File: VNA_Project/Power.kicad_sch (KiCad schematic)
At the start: 33 parts, among them J201 USB_C_Receptacle_USB2.0_16P, J202 Jack-DC, U201 AP7375, U202 USBLC6-2SC6, U203 TLV62569DBV, U204 HT7533-1

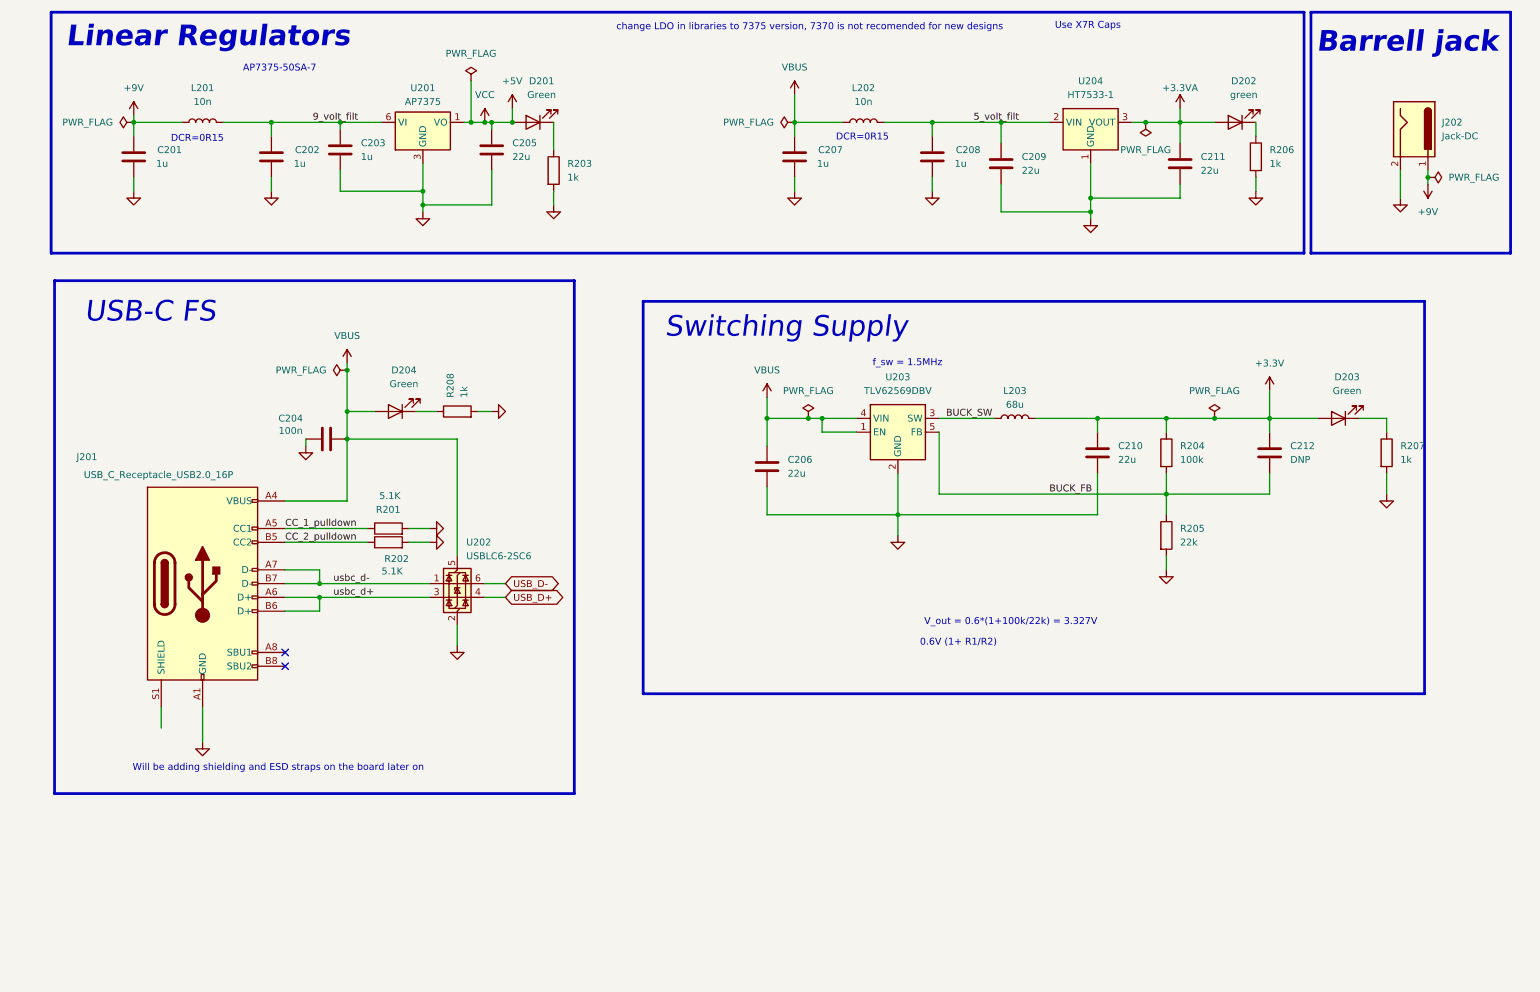
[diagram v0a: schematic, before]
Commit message: adc
adc
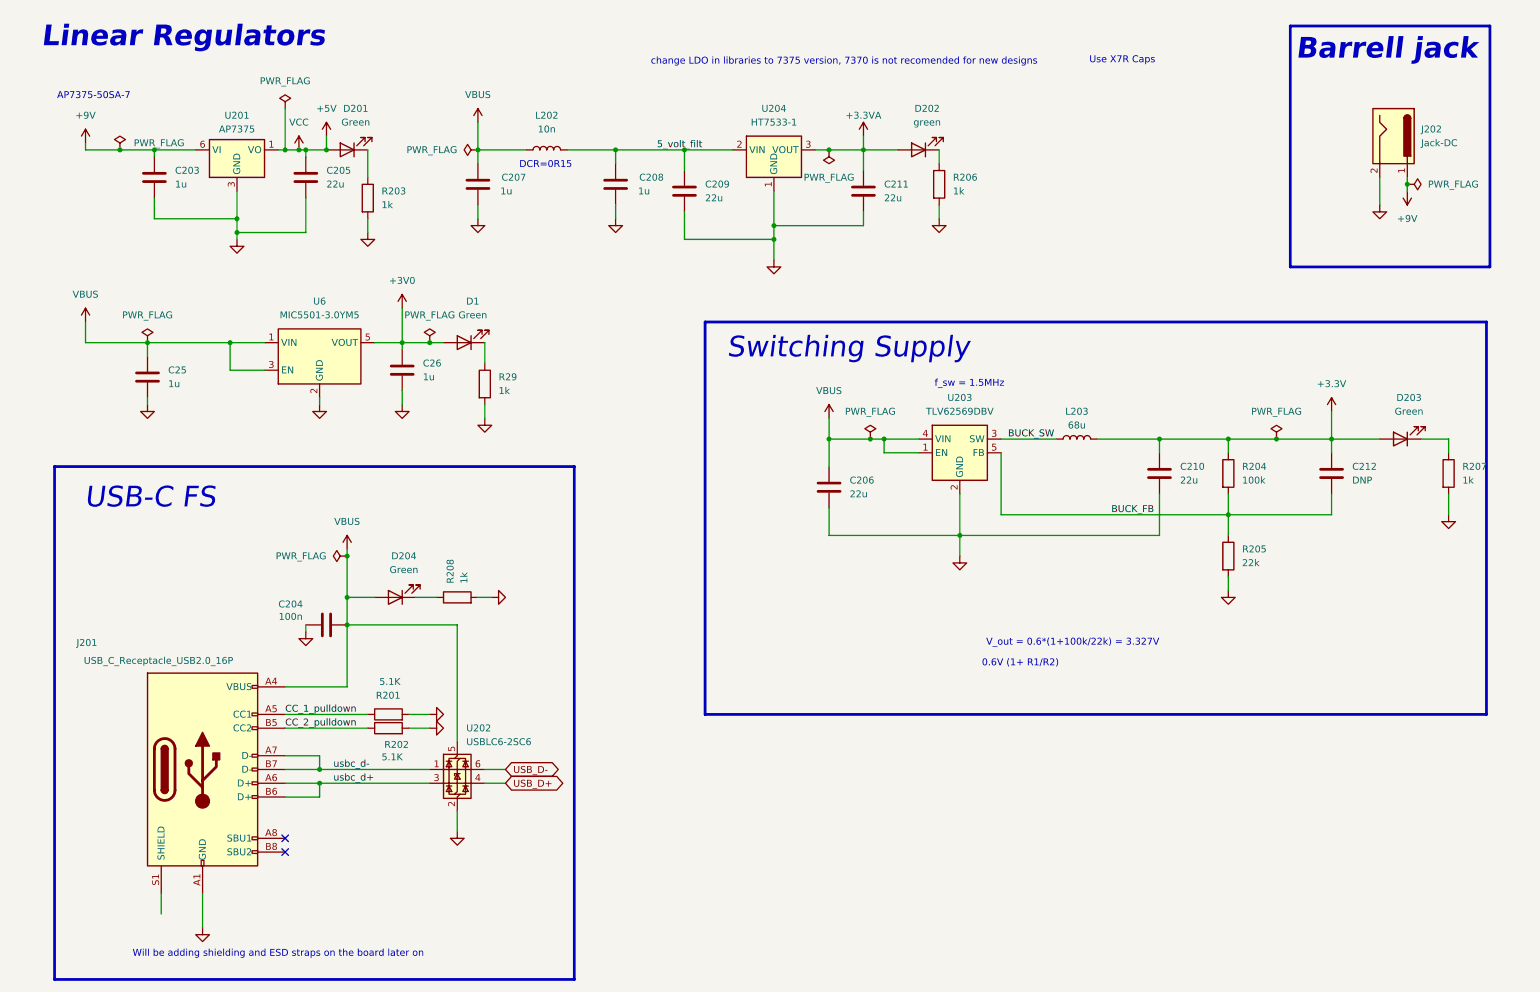
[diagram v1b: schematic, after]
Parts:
- removed C201, C202: 1u, Capacitor_SMD:C_0603_1608Metric, symbol Device:C
- removed L201: 10n, Inductor_SMD:L_0402_1005Metric, symbol Device:L
- added C25, C26: 1u, symbol Device:C
- added D1: Green, symbol Device:LED
- added R29: 1k, symbol Device:R
- added U6: MIC5501-3.0YM5, Package_TO_SOT_SMD:SOT-23-5, symbol Regulator_Linear:MIC5501-3.0YM5
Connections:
- net 9_volt_filt is gone; now on net +9V: C203.1, U201.6 (VI)
- net GND: now also C25.2, C26.2, R29.2, U6.2 (GND)
- net VBUS: now also C25.1, U6.1 (VIN), U6.3 (EN)
- new net: D1.1 (K), R29.1
- new net +3V0: C26.1, D1.2 (A), U6.5 (VOUT)
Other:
- moved on the sheet: C203, C204, C205, C206, C207, C208, C209, C210, C211, C212, D201, D202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
